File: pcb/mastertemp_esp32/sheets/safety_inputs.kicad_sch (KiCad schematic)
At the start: 5 parts, among them J3 SAFETY_STACK_MANUAL_ORDER, U10 STATIC_SAFETY_GATE_TBD

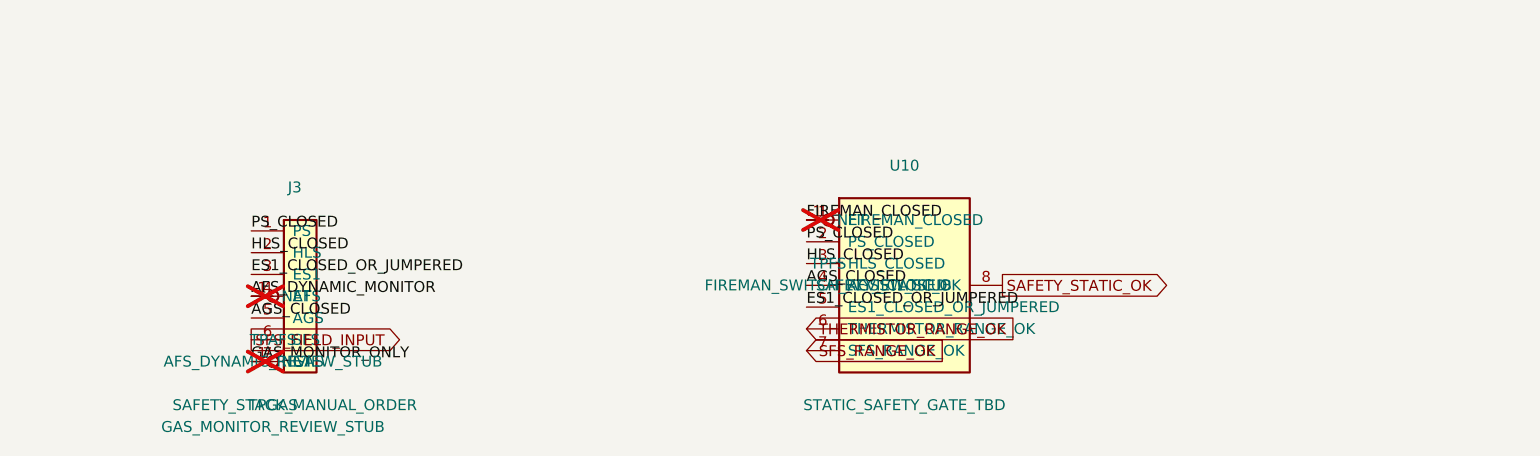
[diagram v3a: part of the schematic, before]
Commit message: AI
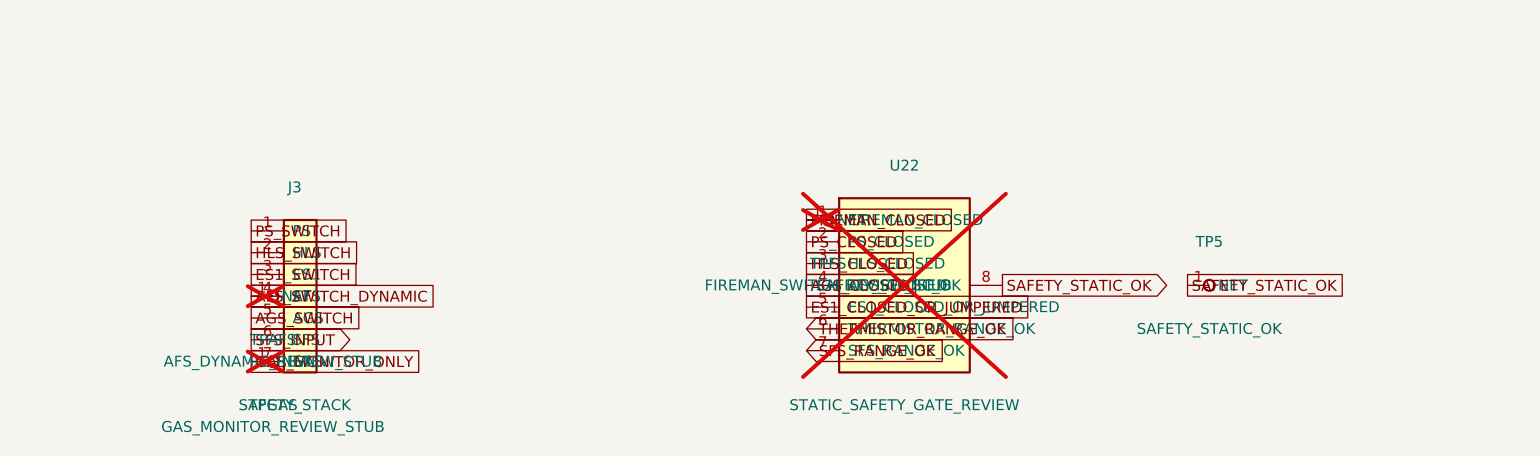
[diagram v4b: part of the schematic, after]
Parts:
- added TP5: SAFETY_STATIC_OK, TestPoint_Pad_D2.0mm, symbol mastertemp_esp32:NetStub_1pin
- J3: value SAFETY_STACK_MANUAL_ORDER -> SAFETY_STACK; footprint TerminalBlock_Phoenix:PhoenixContact_MSTBA_2,5_7-G-5,08_1x07_P5.08mm_Horizontal -> Connector_Phoenix_MSTB:PhoenixContact_MSTBA_2,5_7-G-5,08_1x07_P5.08mm_Horizontal
- U22: renamed from U10; value STATIC_SAFETY_GATE_TBD -> STATIC_SAFETY_GATE_REVIEW; now not fitted; now left out of the parts list
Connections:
- net AGS_CLOSED: no longer J3.5 (AGS)
- net ES1_CLOSED_OR_JUMPERED: no longer J3.3 (ES1)
- net HLS_CLOSED: no longer J3.2 (HLS)
- net PS_CLOSED: no longer J3.1 (PS)
- net SAFETY_STATIC_OK: now also TP5.1 (NET)
- net AFS_DYNAMIC_MONITOR renamed AFS_SWITCH_DYNAMIC
- net SFS_FIELD_INPUT renamed SFS_INPUT
- new net AGS_SWITCH: J3.5 (AGS)
- new net ES1_SWITCH: J3.3 (ES1)
- new net HLS_SWITCH: J3.2 (HLS)
- new net PS_SWITCH: J3.1 (PS)
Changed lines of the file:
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@@
     (dnp no)
     (property "Reference" "J3" (at 71.12 139.7 0) (effects (font (size 1.27 1.27))))
-    (property "Value" "SAFETY_STACK_MANUAL_ORDER" (at 71.12 165.1 0) (effects (font (size 1.27 1.27))))
-    (property "Footprint" "TerminalBlock_Phoenix:PhoenixContact_MSTBA_2,5_7-G-5,08_1x07_P5.08mm_Horizontal" (at 71.12 152.4 0) (effects (font (size 1.27 1.27)) (hide yes)))
+    (property "Value" "SAFETY_STACK" (at 71.12 165.1 0) (effects (font (size 1.27 1.27))))
+    (property "Footprint" "Connector_Phoenix_MSTB:PhoenixContact_MSTBA_2,5_7-G-5,08_1x07_P5.08mm_Horizontal" (at 71.12 152.4 0) (effects (font (size 1.27 1.27)) (hide yes)))
     (property "Datasheet" "~" (at 71.12 152.4 0) (effects (font (size 1.27 1.27)) (hide yes)))
     (property "Description" "Manual Rev. C Figure 24 safety stack terminals" (at 71.12 152.4 0) (effects (font (size 1.27 1.27)) (hide yes)))
@@
     (unit 1)
     (exclude_from_sim no)
-    (in_bom yes)
-    (on_board yes)
-    (dnp no)
-    (property "Reference" "U10" (at 142.24 137.16 0) (effects (font (size 1.27 1.27))))
-    (property "Value" "STATIC_SAFETY_GATE_TBD" (at 142.24 165.1 0) (effects (font (size 1.27 1.27))))
+    (in_bom no)
+    (on_board no)
+    (dnp yes)
+    (property "Reference" "U22" (at 142.24 137.16 0) (effects (font (size 1.27 1.27))))
+    (property "Value" "STATIC_SAFETY_GATE_REVIEW" (at 142.24 165.1 0) (effects (font (size 1.27 1.27))))
     (property "Footprint" "" (at 142.24 151.13 0) (effects (font (size 1.27 1.27)) (hide yes)))
     (property "Datasheet" "~" (at 142.24 151.13 0) (effects (font (size 1.27 1.27)) (hide yes)))
@@
     (pin "7")
     (pin "8")
-    (instances (project "mastertemp_esp32" (path "/82ec6d80-25f4-4b98-986b-98eab22f32ad" (reference "U10") (unit 1))))
+    (instances (project "mastertemp_esp32" (path "/82ec6d80-25f4-4b98-986b-98eab22f32ad" (reference "U22") (unit 1))))
   )
-  (label "PS_CLOSED" (at 66.04 144.78 0) (fields_autoplaced yes) (effects (font (size 1.27 1.27)) (justify left bottom)))
-  (label "HLS_CLOSED" (at 66.04 147.32 0) (fields_autoplaced yes) (effects (font (size 1.27 1.27)) (justify left bottom)))
-  (label "ES1_CLOSED_OR_JUMPERED" (at 66.04 149.86 0) (fields_autoplaced yes) (effects (font (size 1.27 1.27)) (justify left bottom)))
-  (label "AFS_DYNAMIC_MONITOR" (at 66.04 152.4 0) (fields_autoplaced yes) (effects (font (size 1.27 1.27)) (justify left bottom)))
-  (label "AGS_CLOSED" (at 66.04 154.94 0) (fields_autoplaced yes) (effects (font (size 1.27 1.27)) (justify left bottom)))
-  (global_label "SFS_FIELD_INPUT" (shape output) (at 66.04 157.48 0) (fields_autoplaced yes) (effects (font (size 1.27 1.27)) (justify left bottom)))
-  (label "GAS_MONITOR_ONLY" (at 66.04 160.02 0) (fields_autoplaced yes) (effects (font (size 1.27 1.27)) (justify left bottom)))
-  (label "FIREMAN_CLOSED" (at 130.81 143.51 0) (fields_autoplaced yes) (effects (font (size 1.27 1.27)) (justify left bottom)))
-  (label "PS_CLOSED" (at 130.81 146.05 0) (fields_autoplaced yes) (effects (font (size 1.27 1.27)) (justify left bottom)))
-  (label "HLS_CLOSED" (at 130.81 148.59 0) (fields_autoplaced yes) (effects (font (size 1.27 1.27)) (justify left bottom)))
-  (label "AGS_CLOSED" (at 130.81 151.13 0) (fields_autoplaced yes) (effects (font (size 1.27 1.27)) (justify left bottom)))
-  (label "ES1_CLOSED_OR_JUMPERED" (at 130.81 153.67 0) (fields_autoplaced yes) (effects (font (size 1.27 1.27)) (justify left bottom)))
+  (global_label "PS_SWITCH"
+    (shape passive)
+    (at 66.04 144.78 0) (fields_autoplaced yes) (effects (font (size 1.27 1.27)) (justify left bottom))
+  )
+  (global_label "HLS_SWITCH"
+    (shape passive)
+    (at 66.04 147.32 0) (fields_autoplaced yes) (effects (font (size 1.27 1.27)) (justify left bottom))
+  )
+  (global_label "ES1_SWITCH"
+    (shape passive)
+    (at 66.04 149.86 0) (fields_autoplaced yes) (effects (font (size 1.27 1.27)) (justify left bottom))
+  )
+  (global_label "AFS_SWITCH_DYNAMIC"
+    (shape passive)
+    (at 66.04 152.4 0) (fields_autoplaced yes) (effects (font (size 1.27 1.27)) (justify left bottom))
+  )
+  (global_label "AGS_SWITCH"
+    (shape passive)
+    (at 66.04 154.94 0) (fields_autoplaced yes) (effects (font (size 1.27 1.27)) (justify left bottom))
+  )
+  (global_label "SFS_INPUT" (shape output) (at 66.04 157.48 0) (fields_autoplaced yes) (effects (font (size 1.27 1.27)) (justify left bottom)))
+  (global_label "GAS_MONITOR_ONLY"
+    (shape passive)
+    (at 66.04 160.02 0) (fields_autoplaced yes) (effects (font (size 1.27 1.27)) (justify left bottom))
+  )
+  (global_label "FIREMAN_CLOSED"
+    (shape passive)
+    (at 130.81 143.51 0) (fields_autoplaced yes) (effects (font (size 1.27 1.27)) (justify left bottom))
+  )
+  (global_label "PS_CLOSED"
+    (shape passive)
+    (at 130.81 146.05 0) (fields_autoplaced yes) (effects (font (size 1.27 1.27)) (justify left bottom))
+  )
+  (global_label "HLS_CLOSED"
+    (shape passive)
+    (at 130.81 148.59 0) (fields_autoplaced yes) (effects (font (size 1.27 1.27)) (justify left bottom))
+  )
+  (global_label "AGS_CLOSED"
+    (shape passive)
+    (at 130.81 151.13 0) (fields_autoplaced yes) (effects (font (size 1.27 1.27)) (justify left bottom))
+  )
+  (global_label "ES1_CLOSED_OR_JUMPERED"
+    (shape passive)
+    (at 130.81 153.67 0) (fields_autoplaced yes) (effects (font (size 1.27 1.27)) (justify left bottom))
+  )
   (global_label "THERMISTOR_RANGE_OK" (shape input) (at 130.81 156.21 0) (fields_autoplaced yes) (effects (font (size 1.27 1.27)) (justify left bottom)))
   (global_label "SFS_RANGE_OK" (shape input) (at 130.81 158.75 0) (fields_autoplaced yes) (effects (font (size 1.27 1.27)) (justify left bottom)))
@@
     (instances (project "mastertemp_esp32" (path "/82ec6d80-25f4-4b98-986b-98eab22f32ad" (reference "TPFS") (unit 1))))
   )
+  (symbol
+    (lib_id "mastertemp_esp32:NetStub_1pin")
+    (at 177.8 151.13 0)
+    (unit 1)
+    (exclude_from_sim yes)
+    (in_bom no)
+    (on_board yes)
+    (dnp no)
+    (property "Reference" "TP5" (at 177.8 146.05 0) (effects (font (size 1.27 1.27))))
+    (property "Value" "SAFETY_STATIC_OK" (at 177.8 156.21 0) (effects (font (size 1.27 1.27))))
+    (property "Footprint" "TestPoint_Pad_D2.0mm" (at 177.8 151.13 0) (effects (font (size 1.27 1.27)) (hide yes)))
+    (property "Datasheet" "~" (at 177.8 151.13 0) (effects (font (size 1.27 1.27)) (hide yes)))
+    (property "Description" "PCB test point for static safety OK" (at 177.8 151.13 0) (effects (font (size 1.27 1.27)) (hide yes)))
+    (pin "1")
+    (instances (project "mastertemp_esp32" (path "/82ec6d80-25f4-4b98-986b-98eab22f32ad" (reference "TP5") (unit 1))))
+  )
+  (global_label "SAFETY_STATIC_OK" (shape passive) (at 175.26 151.13 0) (fields_autoplaced yes) (effects (font (size 1.27 1.27)) (justify left bottom)))
   (sheet_instances
     (path "/82ec6d80-25f4-4b98-986b-98eab22f32ad" (page "5"))
